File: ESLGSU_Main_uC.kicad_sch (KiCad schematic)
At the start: 46 parts, among them U29 TCAN1051GVDRBRQ, U30 THVD1450DRBR, U31 TMUX1574RSVR, U32 TMUX1574RSVR, U33 TXU0202DTTR, U34 TMUX1574RSVR, U35 TXU0202DTTR, U36 TXB0104RUT, U37 STM32H753ZIT6, U39 PCA9306, U40 TXB0104RUT, U44 TMUX1574RSVR, U46 TXB0104RUT, U47 TMUX1574RSVR

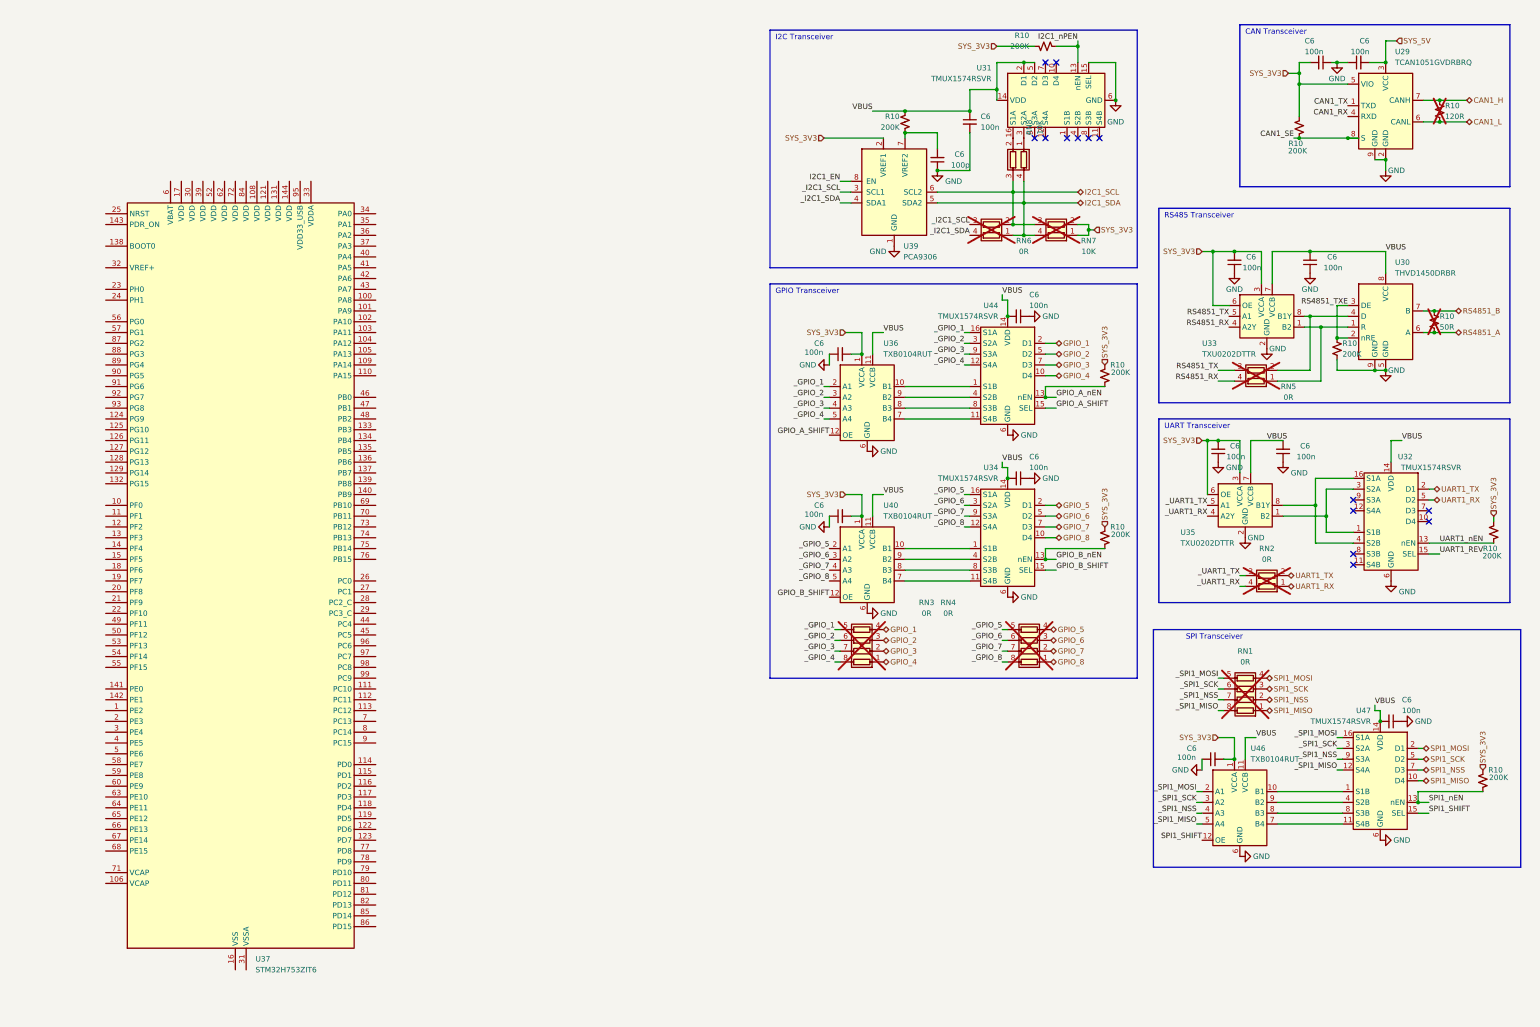
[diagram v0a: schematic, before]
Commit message: Schematic work
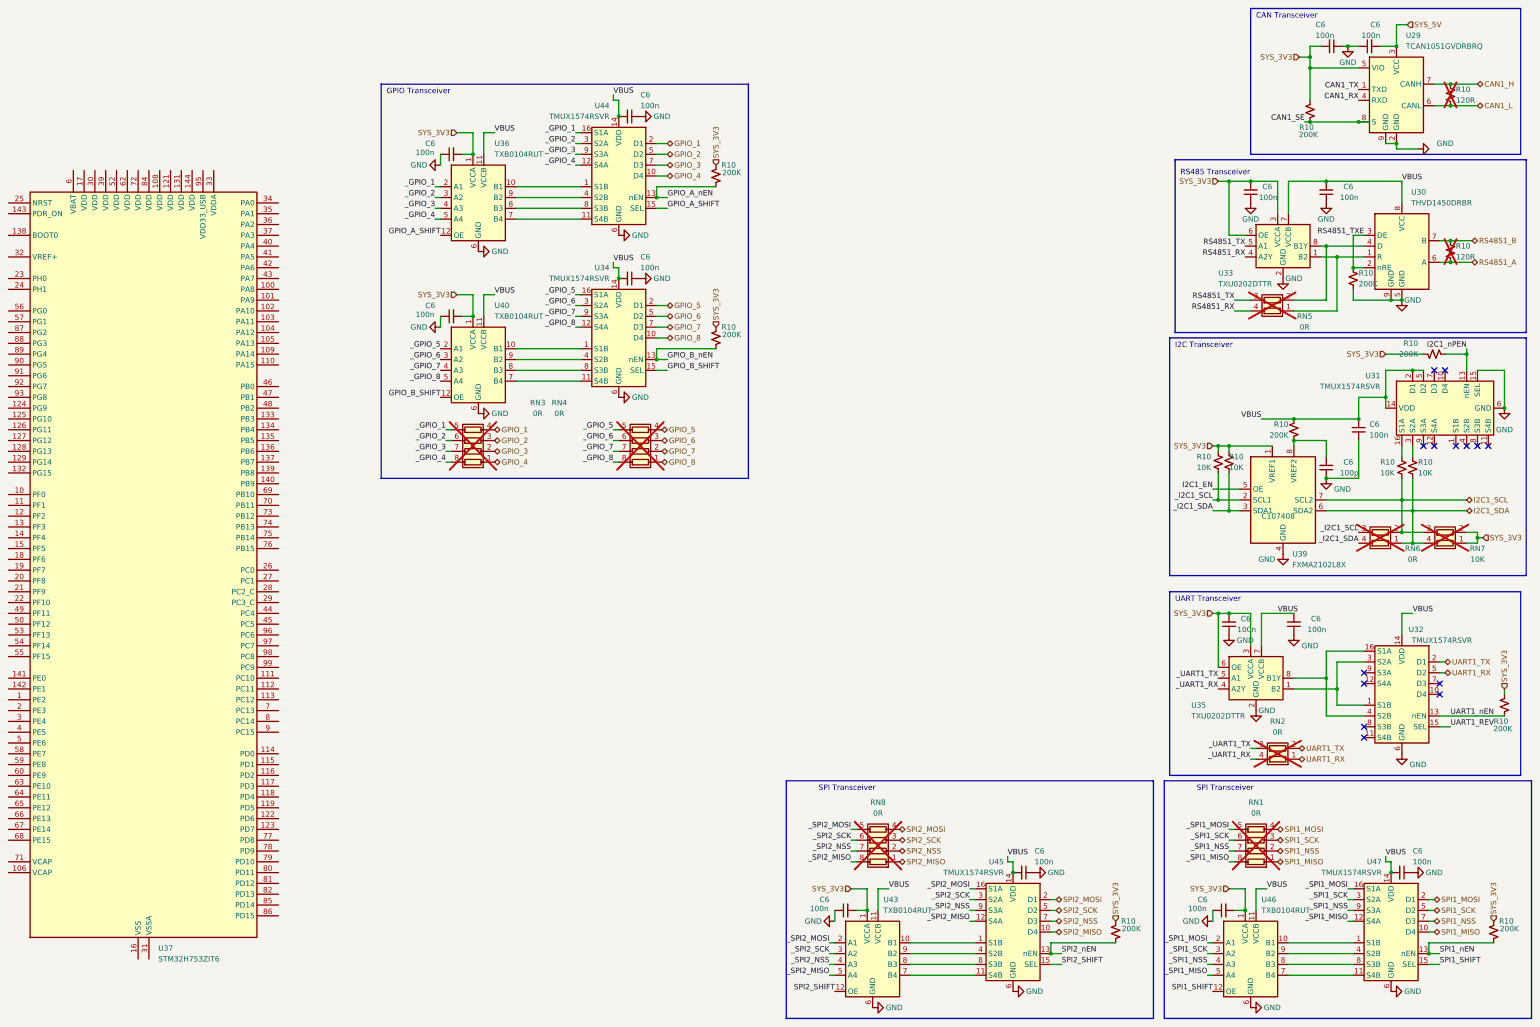
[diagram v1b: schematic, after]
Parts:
- removed R10: 50R, Resistor_SMD:R_0402_1005Metric, symbol Device:R_Small_US
- removed RN8: 10K, Resistor_SMD:R_Array_Convex_2x0402, symbol Device:R_Pack02
- removed U39: PCA9306, ESLGSU_Parts_Lib:SOT833-1-XSON8, symbol Interface:PCA9306
- added C6 (x2): 100n, Capacitor_SMD:C_0402_1005Metric, symbol Device:C_Small
- added R10 (x4): 10K, Resistor_SMD:R_0402_1005Metric, symbol Device:R_Small_US
- added R10: 200K, Resistor_SMD:R_0402_1005Metric, symbol Device:R_Small_US
- added R10: 120R, Resistor_SMD:R_0805_2012Metric, symbol Device:R_Small_US
- added RN8: 0R, Resistor_SMD:R_Array_Concave_4x0402, symbol Device:R_Pack04
- added U39: FXMA2102L8X, symbol ESLGSU_Parts_Lib:FXMA2102L8X
- added U43: TXB0104RUT, ESLGSU_Parts_Lib:T-UQFN-12, symbol ESLGSU_Parts_Lib:TXB0104RUTR
- added U45: TMUX1574RSVR, ESLGSU_Parts_Lib:T-UQFN-16, symbol ESLGSU_Parts_Lib:TMUX1574RSVR
- C6: LCSC Part (none) -> C1546
- C6: LCSC Part (none) -> C307331
- R10: LCSC Part (none) -> C25764
- R10: footprint Resistor_SMD:R_0402_1005Metric -> Resistor_SMD:R_0805_2012Metric; JLCPCB BOM (none) -> 0; LCSC Part (none) -> C17437; now left out of the parts list
- RN1, RN3, RN4: JLCPCB BOM (none) -> 0; LCSC Part (none) -> C2001; now left out of the parts list
- RN2, RN5, RN6: JLCPCB BOM (none) -> 0; LCSC Part (none) -> C75375; now left out of the parts list
- RN7: JLCPCB BOM (none) -> 0; LCSC Part (none) -> C695179; now left out of the parts list
- U29: LCSC Part (none) -> C1848110
- U30: LCSC Part (none) -> C1850226
- U31, U32, U34, U44, U47: LCSC Part (none) -> C2673120
- U33, U35: LCSC Part (none) -> C18197534
- U36, U40, U46: LCSC Part (none) -> C105266
- U37: LCSC Part (none) -> C114408
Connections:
- net GND: now also C6.1, C6.1, U39.4 (GND), U43.6 (GND), U45.6 (GND)
- net I2C1_EN: now also U39.5 (OE)
- net I2C1_SCL: now also R10.2, U39.7 (SCL2)
- net I2C1_SDA: now also R10.2, U39.6 (SDA2)
- net RS4851_A: now also R10.2
- net RS4851_B: now also R10.1
- net SYS_3V3: now also C6.2, R10.1, R10.1, R10.2, U39.1 (VREF1), U43.1 (VCCA)
- net VBUS: now also C6.2, U43.11 (VCCB), U45.14 (VDD)
- net _I2C1_SCL: now also R10.2, U39.2 (SCL1)
- net _I2C1_SDA: now also R10.2, U39.3 (SDA1)
- net at C6.2, R10.2: now also U39.8 (VREF2)
- net at U31.3 (S2A): now also R10.1
- net at U31.16 (S1A): now also R10.1
- new net: U43.10 (B1), U45.1 (S1B)
- new net: U43.7 (B4), U45.11 (S4B)
- new net: U43.8 (B3), U45.8 (S3B)
- new net: U43.9 (B2), U45.4 (S2B)
- new net SPI2_MISO: RN8.1 (R1.1), U45.10 (D4)
- new net SPI2_MOSI: RN8.4 (R4.1), U45.2 (D1)
- new net SPI2_NSS: RN8.2 (R2.1), U45.7 (D3)
- new net SPI2_SCK: RN8.3 (R3.1), U45.5 (D2)
- new net SPI2_SHIFT: U43.12 (OE), U45.15 (SEL)
- new net SPI2_nEN: R10.1, U45.13 (nEN)
- new net _SPI2_MISO: RN8.8 (R1.2), U43.5 (A4), U45.12 (S4A)
- new net _SPI2_MOSI: RN8.5 (R4.2), U43.2 (A1), U45.16 (S1A)
- new net _SPI2_NSS: RN8.7 (R2.2), U43.4 (A3), U45.9 (S3A)
- new net _SPI2_SCK: RN8.6 (R3.2), U43.3 (A2), U45.3 (S2A)
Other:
- moved on the sheet: C6, R10, RN1, RN2, RN3, RN4, RN5, RN6, RN7, U29, U30, U31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
